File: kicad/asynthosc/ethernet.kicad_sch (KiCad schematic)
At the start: 4 parts, among them J3 RJ45_LED, U5 LAN8742A, U6 USBLC6-2P6

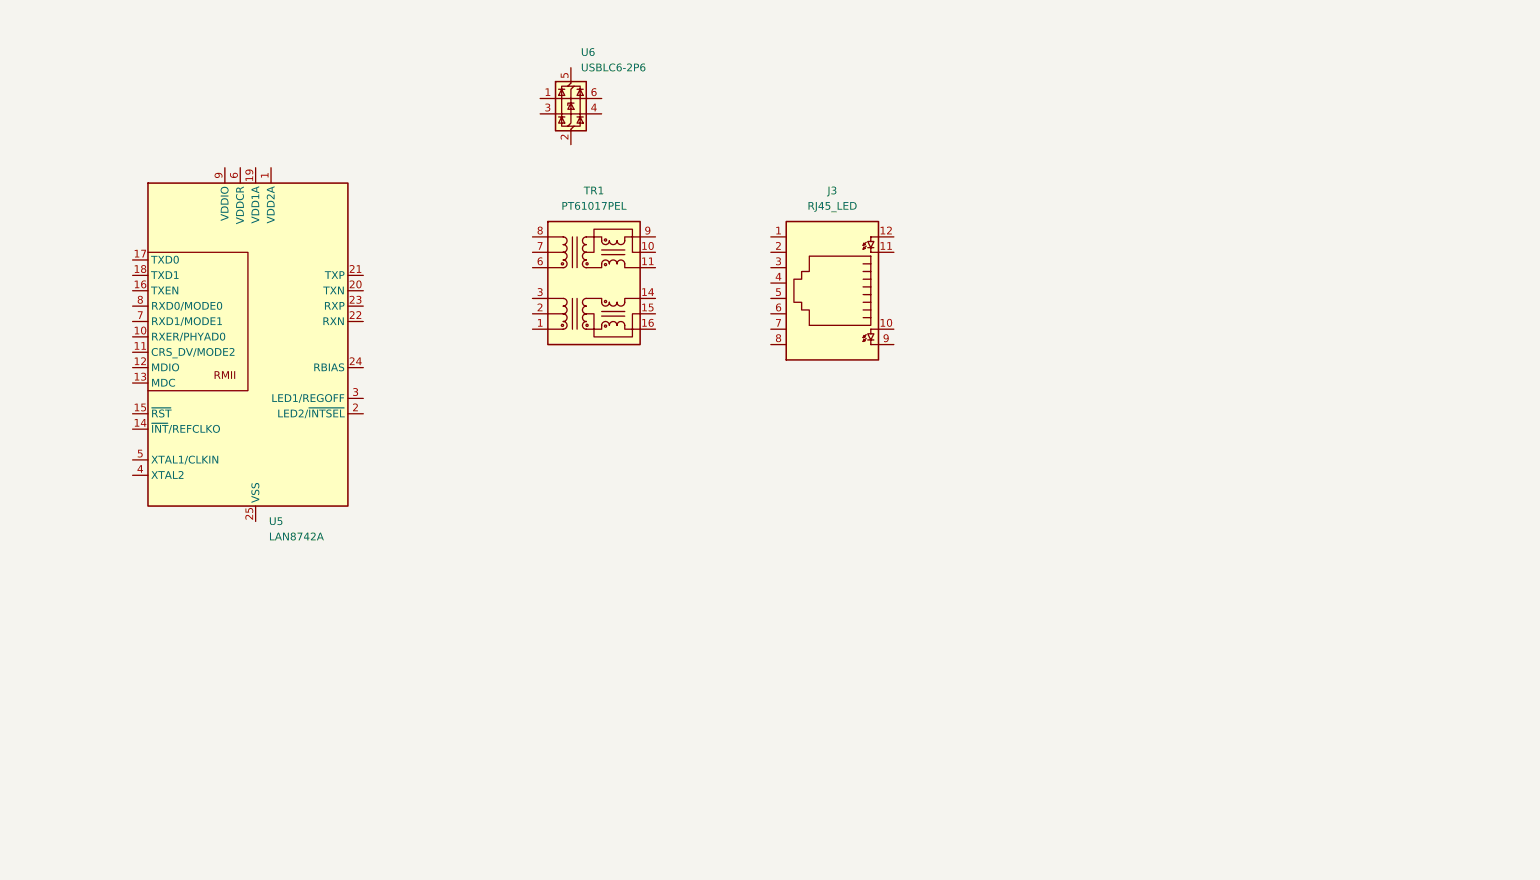
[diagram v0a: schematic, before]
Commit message: sch: rmii side
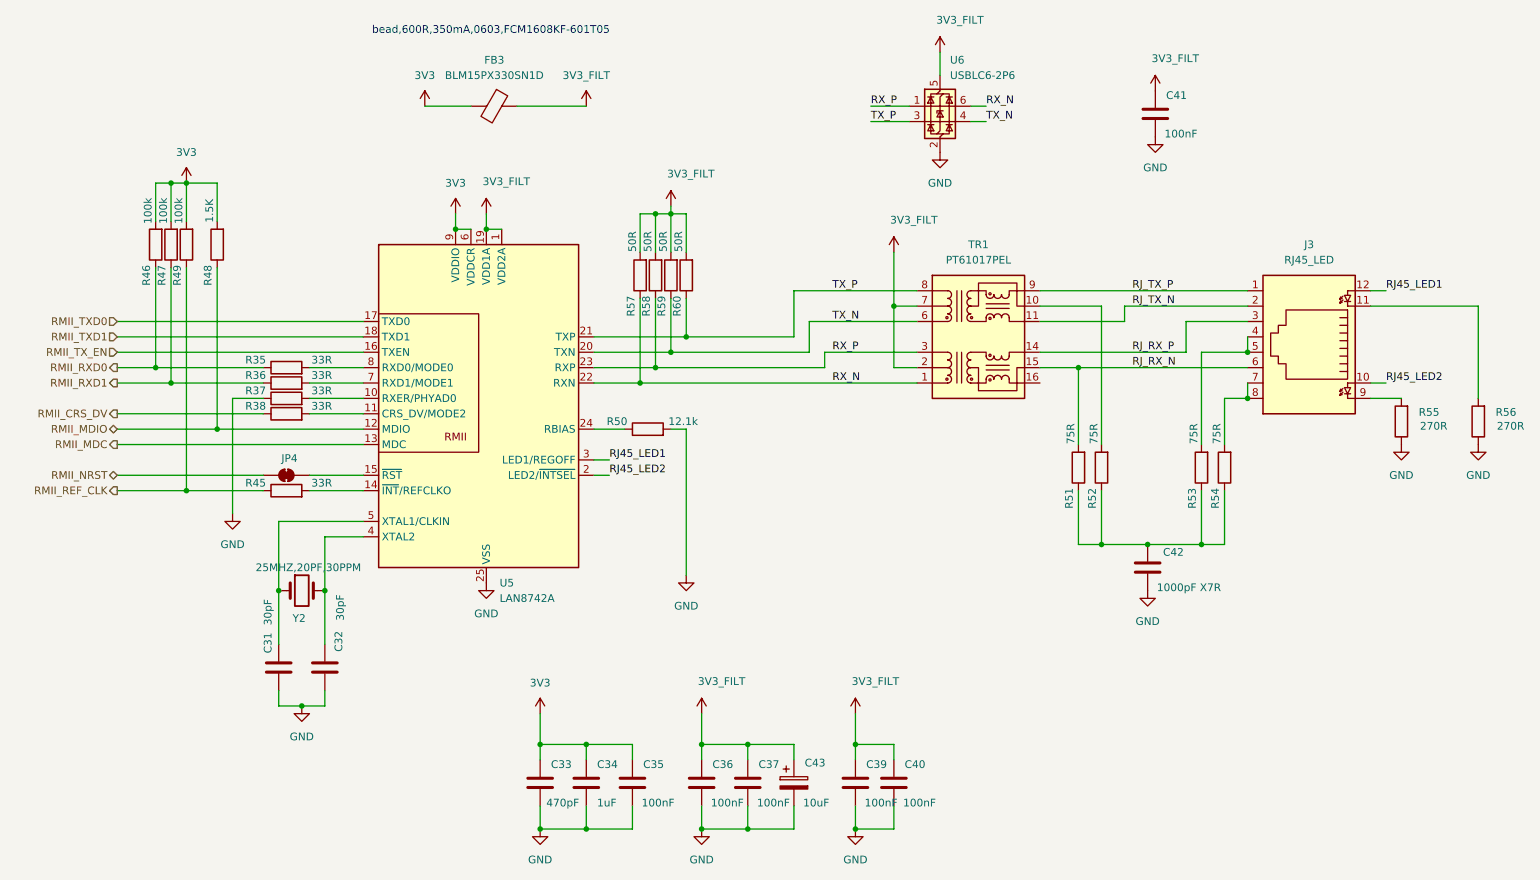
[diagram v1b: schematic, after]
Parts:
- added C31, C32: 30pF, 0402, symbol Device:C
- added C33: 470pF, 0402, symbol Device:C
- added C34: 1uF, 0402, symbol Device:C
- added C35, C36, C37, C39, C40, C41: 100nF, 0402, symbol Device:C
- added C42: 1000pF X7R, 1206, symbol Device:C
- added C43: 10uF, symbol Device:C_Polarized
- added FB3: BLM15PX330SN1D, 0402, symbol Device:FerriteBead
- added JP4: SolderJumper_2_Bridged, symbol Jumper:SolderJumper_2_Bridged
- added R35, R36, R37, R38, R45: 33R, 0402, symbol Device:R
- added R46, R47, R49: 100k, 0402, symbol Device:R
- added R48: 1.5K, 0402, symbol Device:R
- added R50: 12.1k, 0402, symbol Device:R
- added R51, R52, R53, R54: 75R, 0402, symbol Device:R
- added R55, R56: 270R, 0402, symbol Device:R
- added R57, R58, R59, R60: 50R, 0402, symbol Device:R
- added Y2: 25MHZ,20PF,30PPM, symbol Device:Crystal
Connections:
- net RX_P: now reaches U6.1 (I/O1)
- net RX_P: now also TR1.3 (TD-), U5.23 (RXP), R58.1
- net GND: now reaches U6.2 (GND)
- net GND: now also U5.25 (VSS), C31.1, C32.1, C33.2, C34.2, C35.2, C36.2, C37.2, C39.2, C40.2, C41.2, C42.2, C43.2, R37.1, R50.2, R55.1, R56.1
- net TX_P: now reaches U6.3 (I/O2)
- net TX_P: now also TR1.8 (RD-), U5.21 (TXP), R60.1
- net TX_N: now reaches U6.4 (I/O2)
- net TX_N: now also TR1.6 (RD+), U5.20 (TXN), R59.1
- net 3V3_FILT: now reaches U6.5 (VBUS)
- net 3V3_FILT: now also TR1.2 (C_TD), TR1.7 (C_RD), U5.1 (VDD2A), U5.19 (VDD1A), C36.1, C37.1, C39.1, C40.1, C41.1, C43.1, FB3.1, R57.2, R58.2, R59.2, R60.2
- net RX_N: now reaches U6.6 (I/O1)
- net RX_N: now also TR1.1 (TD+), U5.22 (RXN), R57.1
- net RJ_TX_P: now reaches J3.1
- net RJ_TX_P: now also TR1.9 (RX-)
- net RJ45_LED2: now reaches J3.10
- net RJ45_LED2: now also U5.2 (LED2/~{INTSEL})
- net at J3.11: now also R56.2
- net RJ45_LED1: now reaches J3.12
- net RJ45_LED1: now also U5.3 (LED1/REGOFF)
- net RJ_TX_N: now reaches J3.2
- net RJ_TX_N: now also TR1.11 (RX+)
- net RJ_RX_P: now reaches J3.3
- net RJ_RX_P: now also TR1.14 (TX-)
- net at J3.4: now also J3.5, R53.2
- net RJ_RX_N: now reaches J3.6
- net RJ_RX_N: now also TR1.15 (C_TX), R51.2
- net at J3.7: now also J3.8, R54.2
- net at J3.9: now also R55.2
- net at TR1.10 (C_RX): now also R52.2
- net at U5.10 (RXER/PHYAD0): now also R37.2
- net at U5.11 (CRS_DV/MODE2): now also R38.2
- net RMII_MDIO: now reaches U5.12 (MDIO)
- net RMII_MDIO: now also R48.1
- net RMII_MDC: now reaches U5.13 (MDC)
- net at U5.14 (~{INT}/REFCLKO): now also R45.2
- net at U5.15 (~{RST}): now also JP4.1 (A)
- net RMII_TX_EN: now reaches U5.16 (TXEN)
- net RMII_TXD0: now reaches U5.17 (TXD0)
- net RMII_TXD1: now reaches U5.18 (TXD1)
- net at U5.24 (RBIAS): now also R50.1
- net at U5.4 (XTAL2): now also C32.2, Y2.2
- net at U5.5 (XTAL1/CLKIN): now also C31.2, Y2.1
- net 3V3: now reaches U5.6 (VDDCR)
- net 3V3: now also U5.9 (VDDIO), C33.1, C34.1, C35.1, FB3.2, R46.2, R47.2, R48.2, R49.2
- net at U5.7 (RXD1/MODE1): now also R36.2
- net at U5.8 (RXD0/MODE0): now also R35.2
- new net: C42.1, R51.1, R52.1, R53.1, R54.1
- new net RMII_CRS_DV: R38.1
- new net RMII_NRST: JP4.2 (B)
- new net RMII_REF_CLK: R45.1, R49.1
- new net RMII_RXD0: R35.1, R46.1
- new net RMII_RXD1: R36.1, R47.1
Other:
- note added: "bead,600R,350mA,0603,FCM1608KF-601T05"
- moved on the sheet: J3, TR1, U5, U6
